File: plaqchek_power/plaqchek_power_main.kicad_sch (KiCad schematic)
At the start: 28 parts, among them U10 LM34601, U12 TPS54202DDC, U15 TPS62175DQC

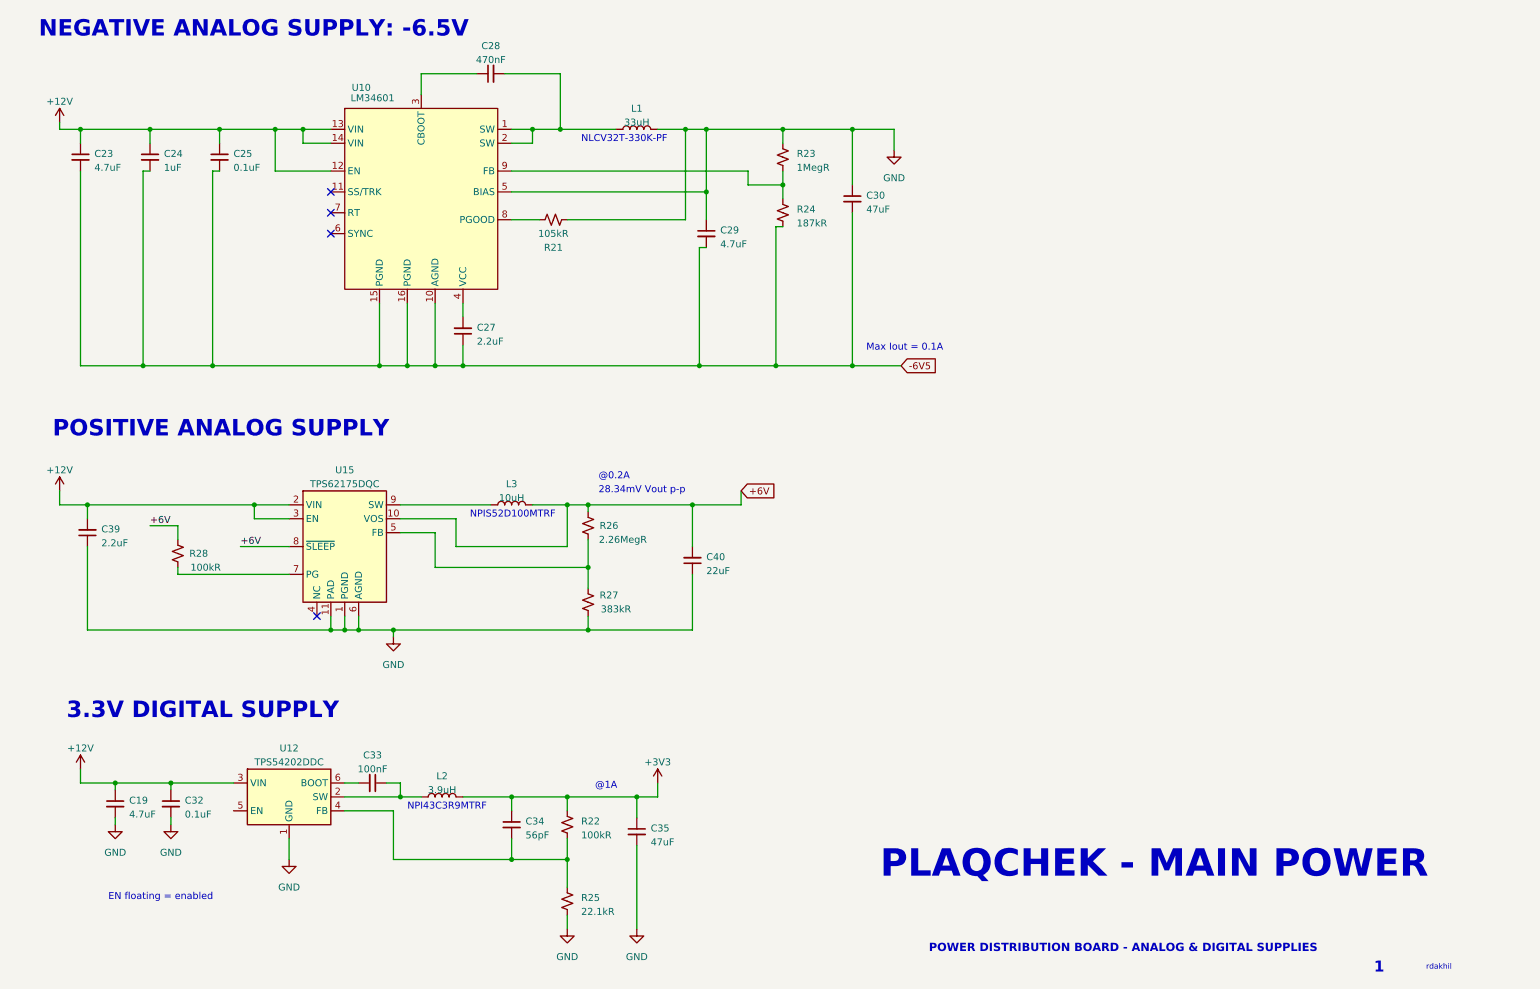
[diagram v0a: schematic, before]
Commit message: finish schematic
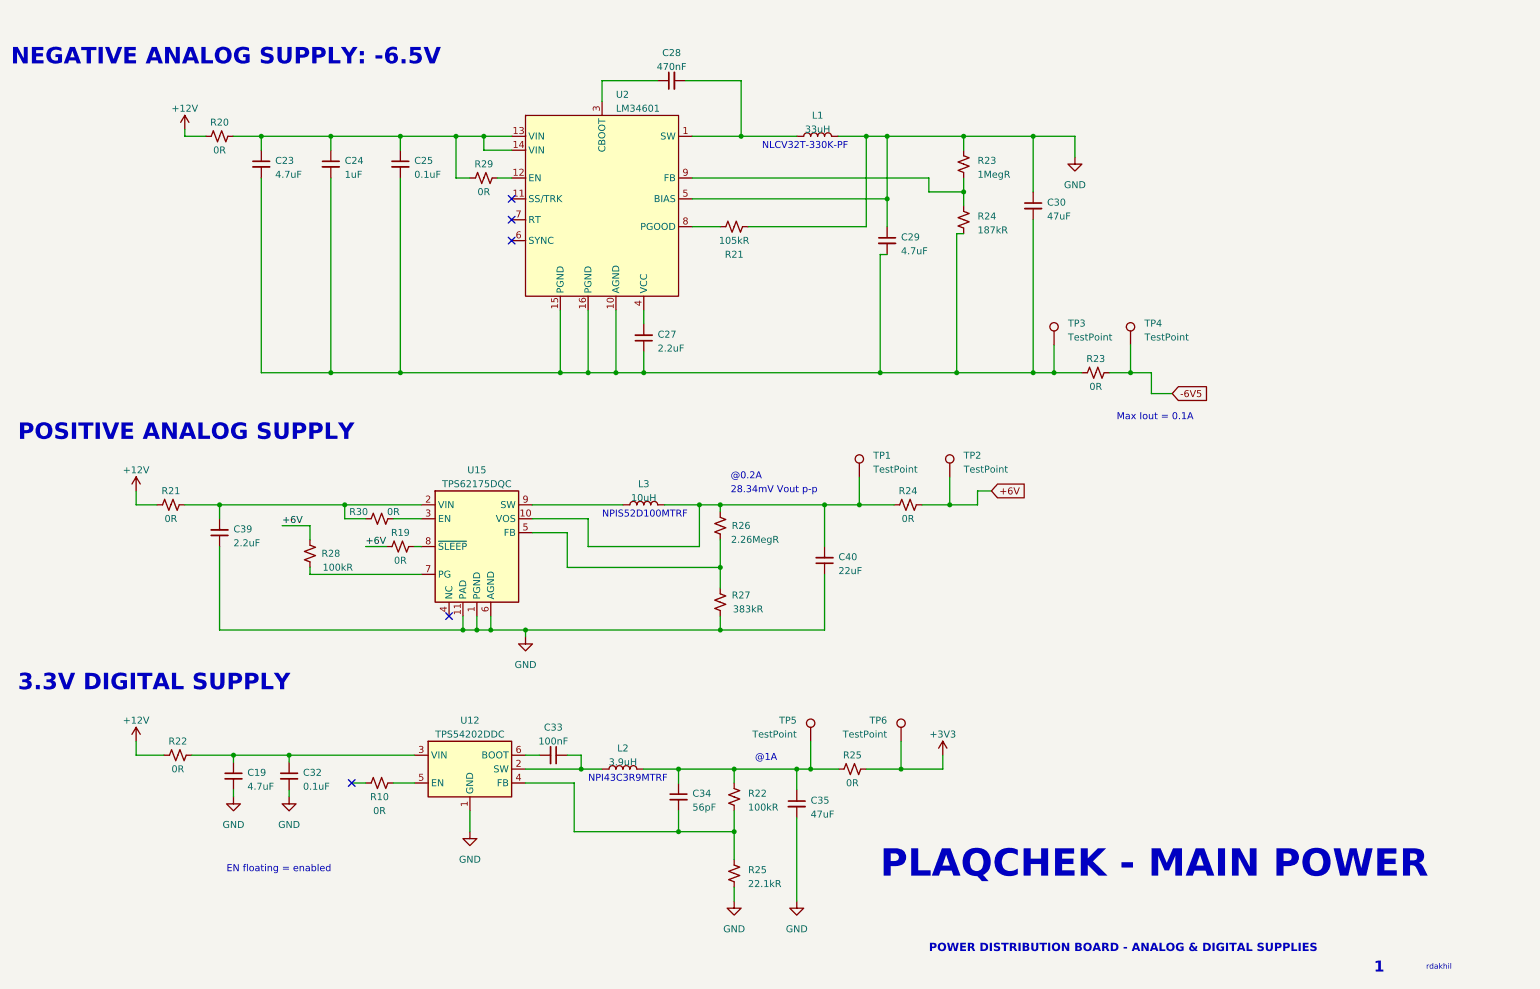
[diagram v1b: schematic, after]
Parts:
- removed U10: LM34601, symbol plaqchek_mlb:LM34601
- added R10, R19, R20, R21, R22, R23, R24, R25, R29, R30: 0R, symbol Device:R_Small_US
- added TP1, TP2, TP3, TP4, TP5, TP6: TestPoint, symbol Connector:TestPoint
- added U2: LM34601, symbol plaqchek:LM34601
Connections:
- net +12V: now also R20.2, R21.2, R22.2; no longer C19.1, C23.1, C24.1, C25.1, C32.1, C39.2, U12.3 (VIN), U15.2 (VIN), U15.3 (EN)
- net +3V3: now also R25.1, TP6.1; no longer C34.1, C35.1, L2.2, R22.1
- net +6V: now also R19.2, R24.1, TP2.1; no longer C40.2, L3.2, R26.1, U15.10 (VOS), U15.8 (~{SLEEP})
- net -6V5: now also R23.1, TP4.1; no longer C23.2, C24.2, C25.2, C27.1, C29.2, C30.2, R24.1
- net GND: now also U2.5 (BIAS)
- net at R23.1, R24.2: now also U2.9 (FB)
- net at U12.5 (EN): now also R10.1
- net at C28.1: now also U2.3 (CBOOT)
- net at C28.2, L1.1: now also U2.1 (SW), U2.2 (SW)
- net at R21.2: now also U2.8 (PGOOD)
- net at C27.2: now also U2.4 (VCC)
- new net: C23.1, C24.1, C25.1, R20.1, R29.2, U2.13 (VIN), U2.14 (VIN)
- new net: C23.2, C24.2, C25.2, C27.1, C29.2, C30.2, R23.2, R24.1, TP3.1, U2.10 (AGND), U2.15 (PGND), U2.16 (PGND)
- new net: C34.1, C35.1, L2.2, R22.1, R25.2, TP5.1
- new net: C19.1, C32.1, R22.1, U12.3 (VIN)
- new net: R19.1, U15.8 (~{SLEEP})
- new net: C39.2, R21.1, R30.1, U15.2 (VIN)
- new net: C40.2, L3.2, R24.2, R26.1, TP1.1, U15.10 (VOS)
- new net: R29.1, U2.12 (EN)
- new net: R30.2, U15.3 (EN)
- no-connect marks 4 -> 5
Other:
- moved on the sheet: C19, C23, C24, C25, C27, C28, C29, C30, C32, C33, C34, C35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
